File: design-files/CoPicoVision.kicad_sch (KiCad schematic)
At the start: 11 parts, among them SW101 SW_Push, U101 Z80CPU, U102 DS1813, U103 74ACT05, X101 3.579545MHZ

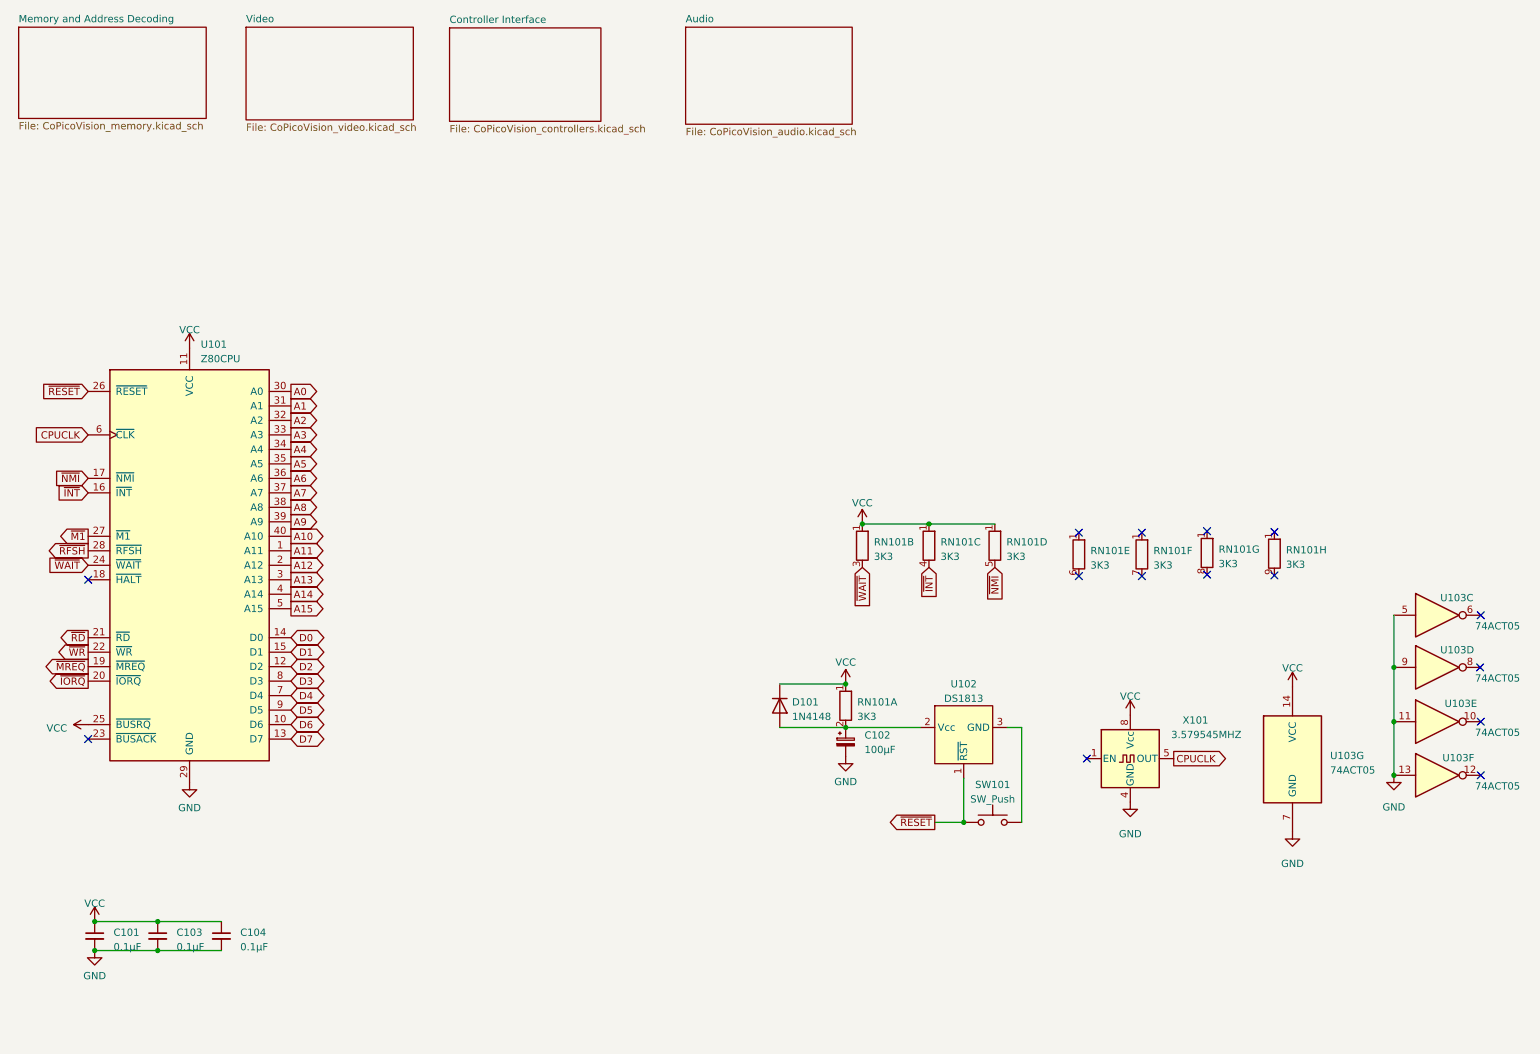
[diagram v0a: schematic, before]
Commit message: Add power supply.  PCB checkpoint.
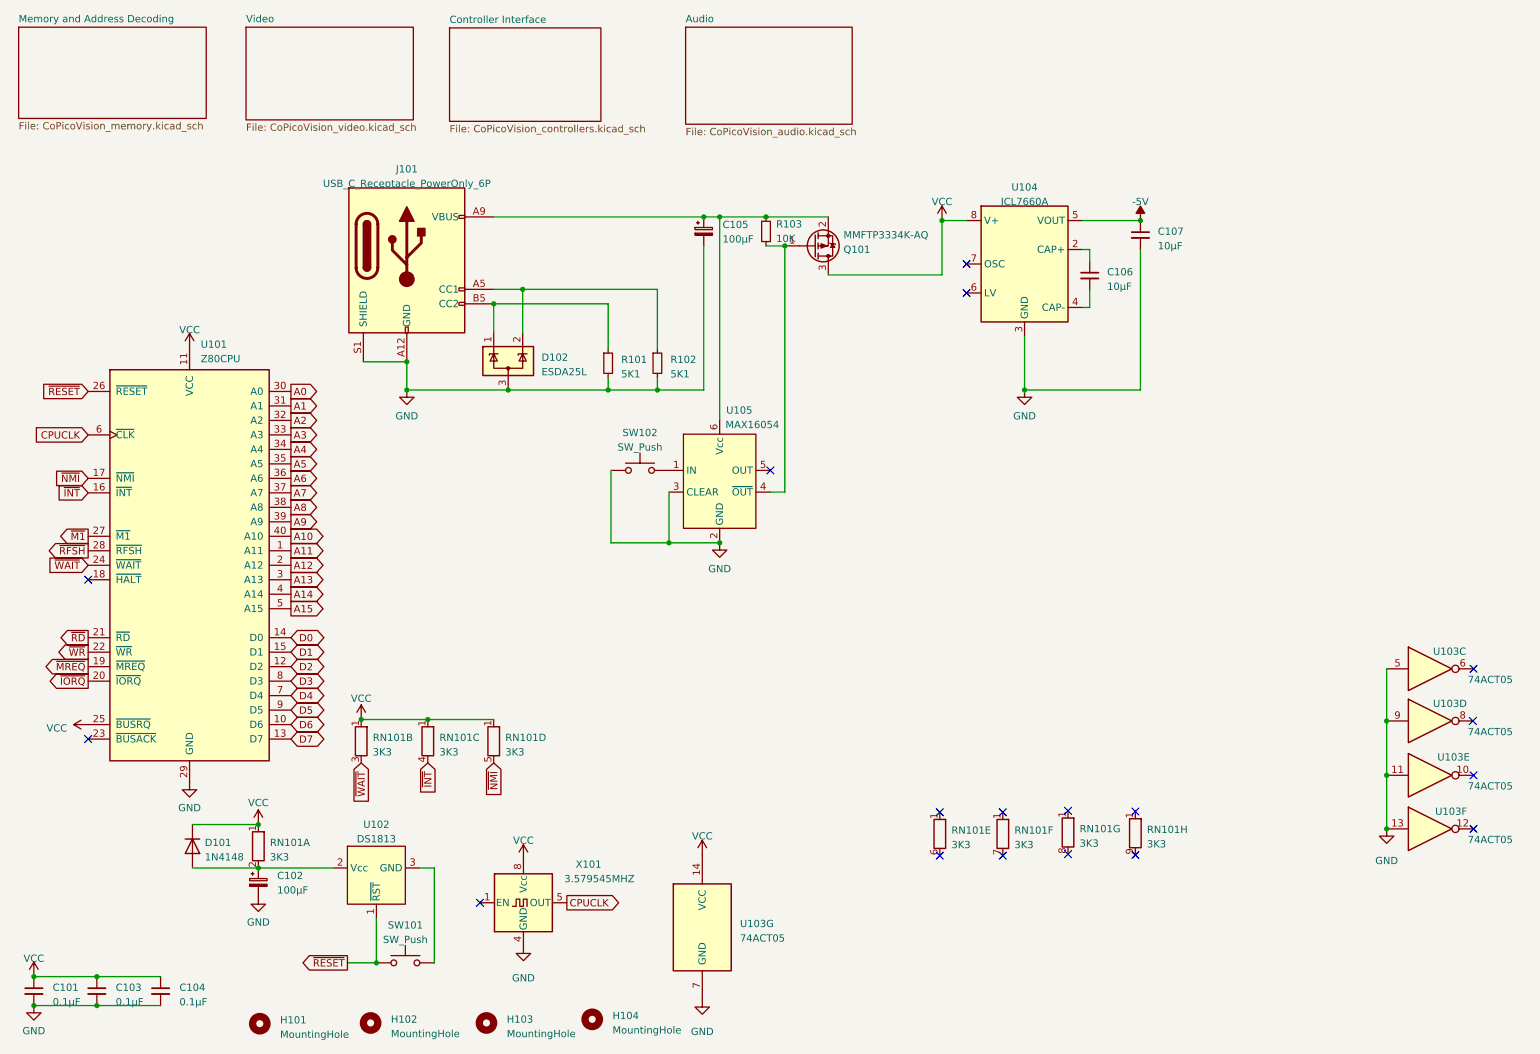
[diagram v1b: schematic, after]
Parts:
- added C105: 100µF, Capacitor_THT:CP_Radial_D6.3mm_P2.50mm, symbol Device:C_Polarized_Small
- added C106, C107: 10µF, Capacitor_SMD:C_0805_2012Metric_Pad1.18x1.45mm_HandSolder, symbol Device:C_Small
- added D102: ESDA25L, Package_TO_SOT_SMD:SOT-23, symbol Power_Protection:SP0502BAHT
- added H101, H102, H103, H104: MountingHole, MountingHole:MountingHole_3.5mm, symbol Mechanical:MountingHole
- added J101: USB_C_Receptacle_PowerOnly_6P, Connector_USB:USB_C_Receptacle_GCT_USB4085, symbol Connector:USB_C_Receptacle_PowerOnly_6P
- added Q101: MMFTP3334K-AQ, Package_TO_SOT_SMD:SOT-23, symbol Device:Q_PMOS_GSD
- added R101, R102: 5K1, Resistor_SMD:R_0805_2012Metric_Pad1.20x1.40mm_HandSolder, symbol Device:R_Small
- added R103: 10K, Resistor_SMD:R_0805_2012Metric_Pad1.20x1.40mm_HandSolder, symbol Device:R_Small
- added SW102: SW_Push, Button_Switch_THT:SW_PUSH_6mm, symbol Switch:SW_Push
- added U104: ICL7660A, Package_SO:SOIC-8_3.9x4.9mm_P1.27mm, symbol Regulator_SwitchedCapacitor:ICL7660
- added U105: MAX16054, Package_TO_SOT_SMD:SOT-23-6, symbol jrt-ICs:MAX16054
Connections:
- net GND: now also C105.2, C107.2, D102.3 (A), J101.A12 (GND), J101.B12 (GND), J101.S1 (SHIELD), R101.2, R102.2, SW102.1, U104.3 (GND), U105.2 (GND), U105.3 (CLEAR)
- net VCC: now also Q101.3 (D), U104.8 (V+)
- new net: C106.1, U104.2 (CAP+)
- new net: C106.2, U104.4 (CAP-)
- new net: C105.1, J101.A9 (VBUS), J101.B9 (VBUS), Q101.2 (S), R103.1, U105.6 (Vcc)
- new net: Q101.1 (G), R103.2, U105.4 (~{OUT})
- new net: D102.1 (K), J101.B5 (CC2), R101.1
- new net: D102.2 (K), J101.A5 (CC1), R102.1
- new net: SW102.2, U105.1 (IN)
- new net -5V: C107.1, U104.5 (VOUT)
- no-connect marks 15 -> 18
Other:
- moved on the sheet: C101, C102, C103, C104, D101, RN101A, RN101B, RN101C, RN101D, RN101E, RN101F, RN101G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
